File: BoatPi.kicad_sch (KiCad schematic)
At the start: 57 parts, among them J1 1432431, J10 CONSMA002-SMD-G, J11 CONSMA002-SMD-G, J12 CONSMA002-SMD-G, J14 Barrel_Jack_MountingPin, J2 1436987, J4 JAE_SIM_Card_SF72S006, J7 1436987, J8 1432431, M2 Fan_CPU_4pin, U1 SIM7600E-H, U10 AP62301WU-7, U2 PC817, U3 PC817, U4 PC817, U5 PC817, U6 PC817, U7 PC817, U8 PC817, U9 PC817

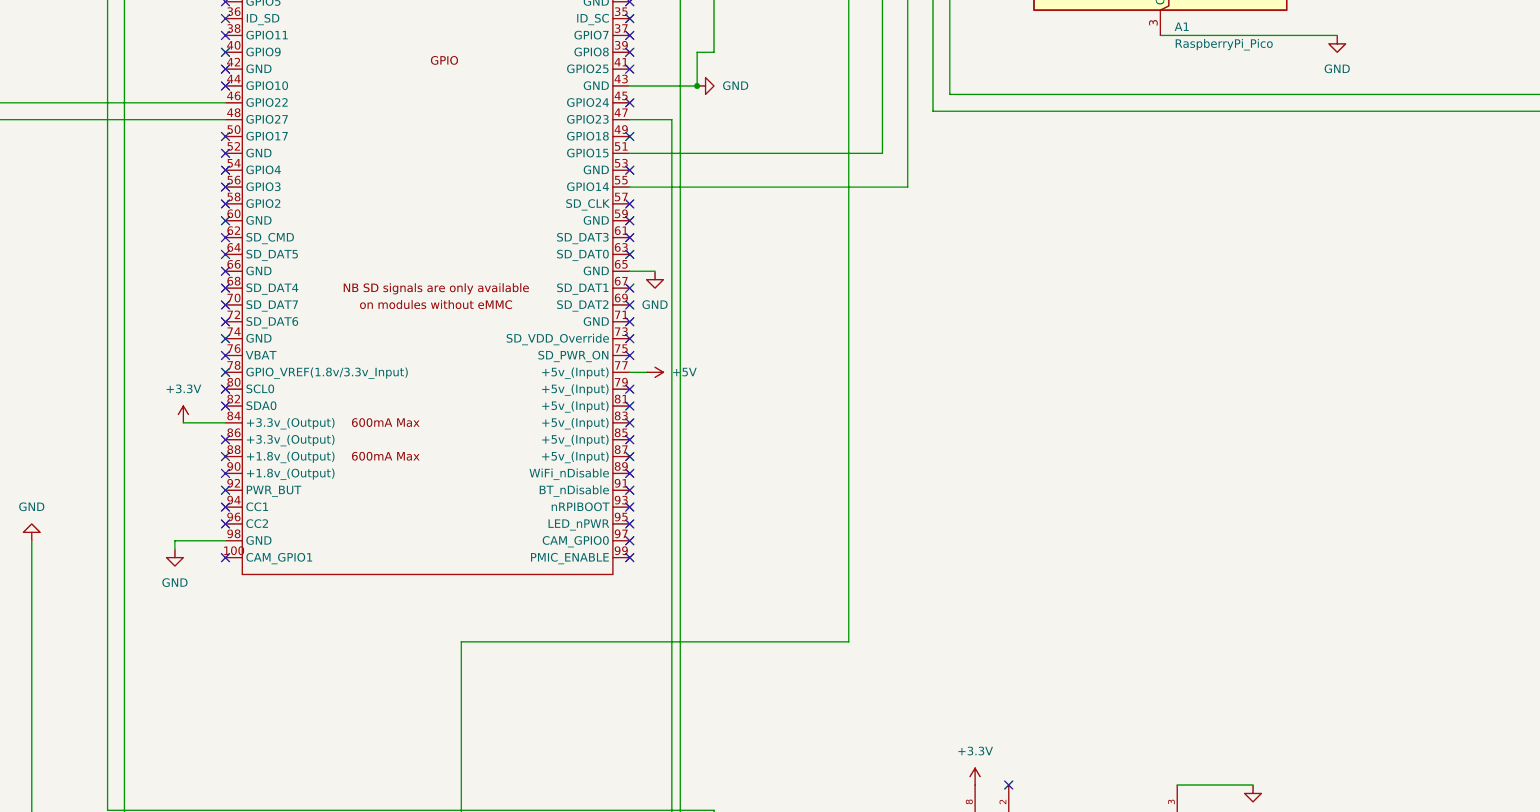
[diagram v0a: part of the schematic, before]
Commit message: Home push
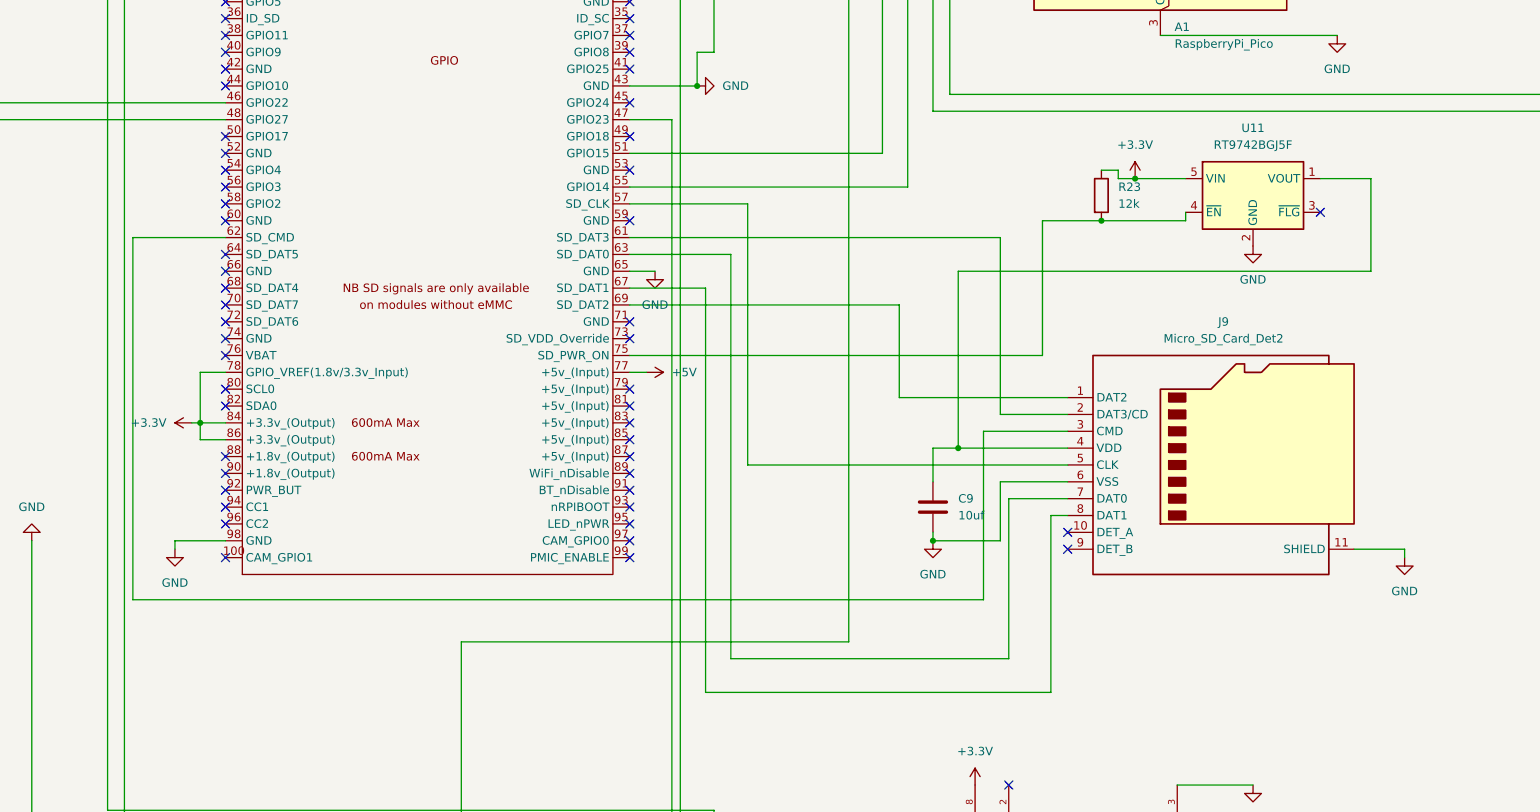
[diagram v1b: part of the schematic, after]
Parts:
- added C9: 10uf, Capacitor_SMD:C_0805_2012Metric, symbol Device:C
- added J9: Micro_SD_Card_Det2, Connector_Card:SD_TE_2041021, symbol Connector:Micro_SD_Card_Det2
- added R23: 12k, Resistor_SMD:R_0805_2012Metric, symbol Device:R
- added U11: RT9742BGJ5F, Package_TO_SOT_SMD:TSOT-23-5, symbol Power_Management:RT9742BGJ5F
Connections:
- net +3.3V: now also Module1.78 (GPIO_VREF(1.8v/3.3v_Input)), Module1.86 (+3.3v_(Output)), R23.1, U11.5 (VIN)
- net GND: now also C9.2, J9.11 (SHIELD), J9.6 (VSS), U11.2 (GND)
- net at Module1.57 (SD_CLK): now also J9.5 (CLK)
- net at Module1.61 (SD_DAT3): now also J9.2 (DAT3/CD)
- net at Module1.62 (SD_CMD): now also J9.3 (CMD)
- net at Module1.63 (SD_DAT0): now also J9.7 (DAT0)
- net at Module1.67 (SD_DAT1): now also J9.8 (DAT1)
- net at Module1.69 (SD_DAT2): now also J9.1 (DAT2)
- net at Module1.75 (SD_PWR_ON): now also R23.2, U11.4 (~{EN})
- new net: C9.1, J9.4 (VDD), U11.1 (VOUT)
- no-connect marks 190 -> 184

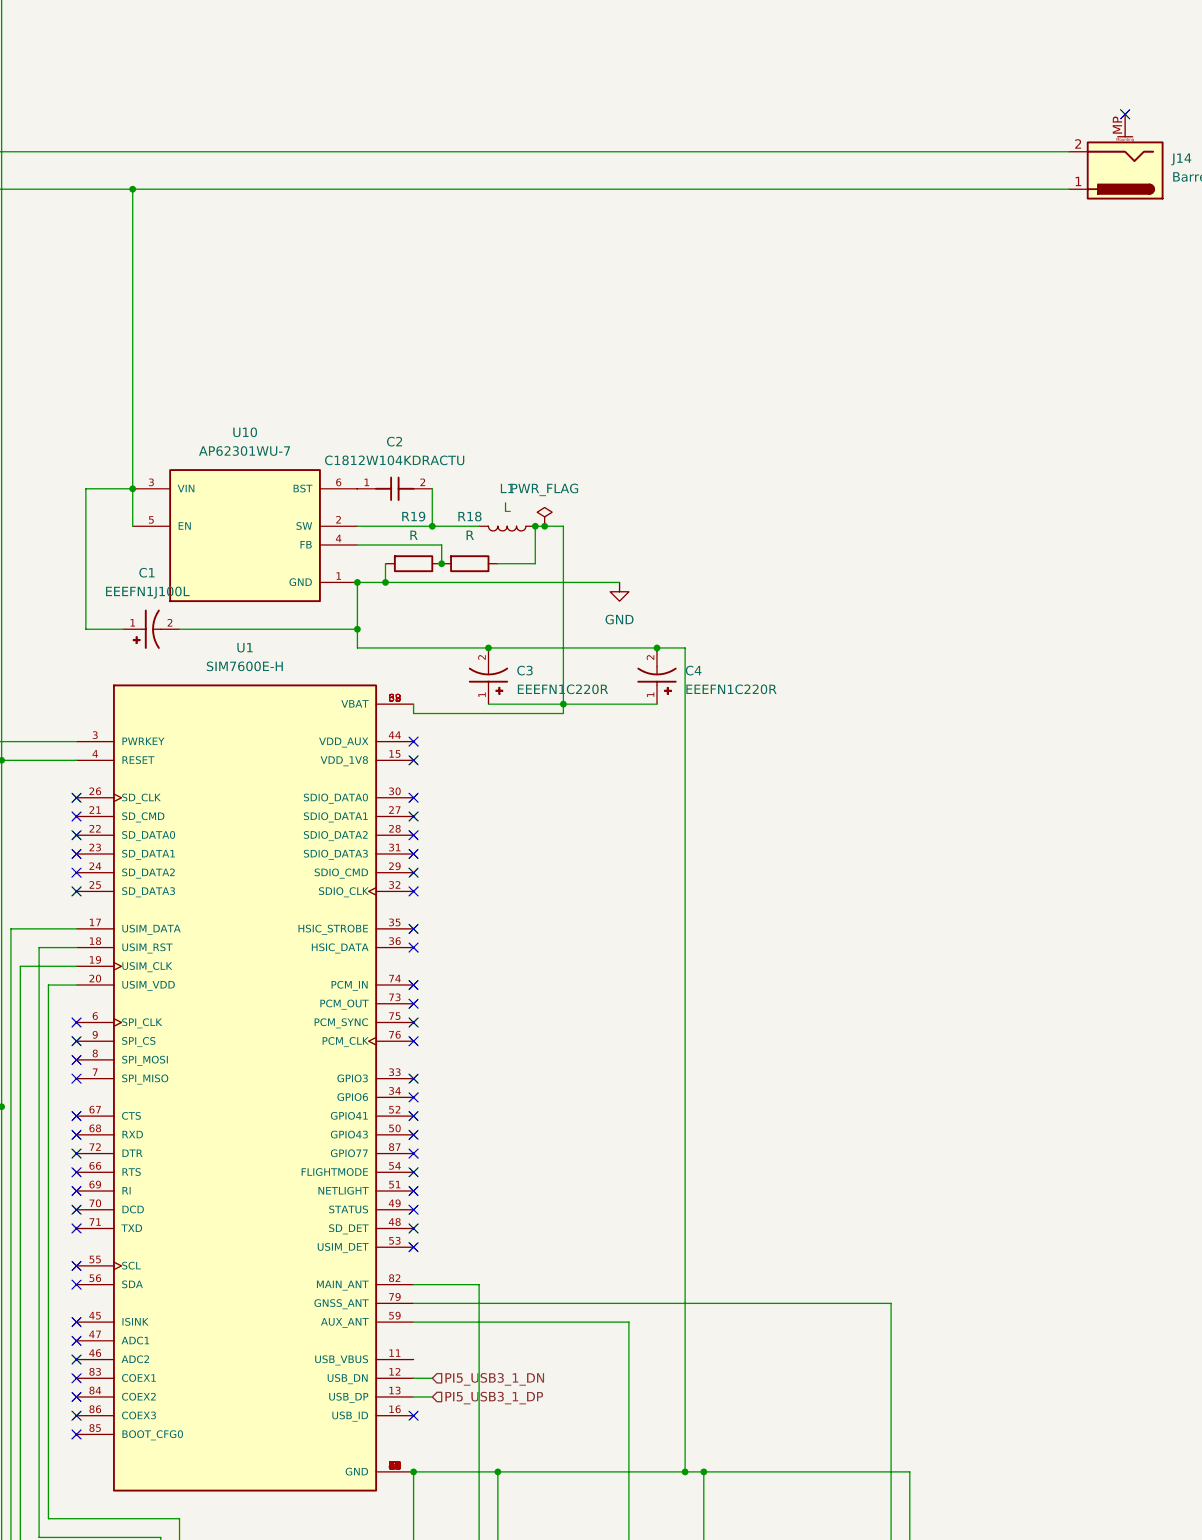
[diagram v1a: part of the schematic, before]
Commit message: Work Changes and documentation
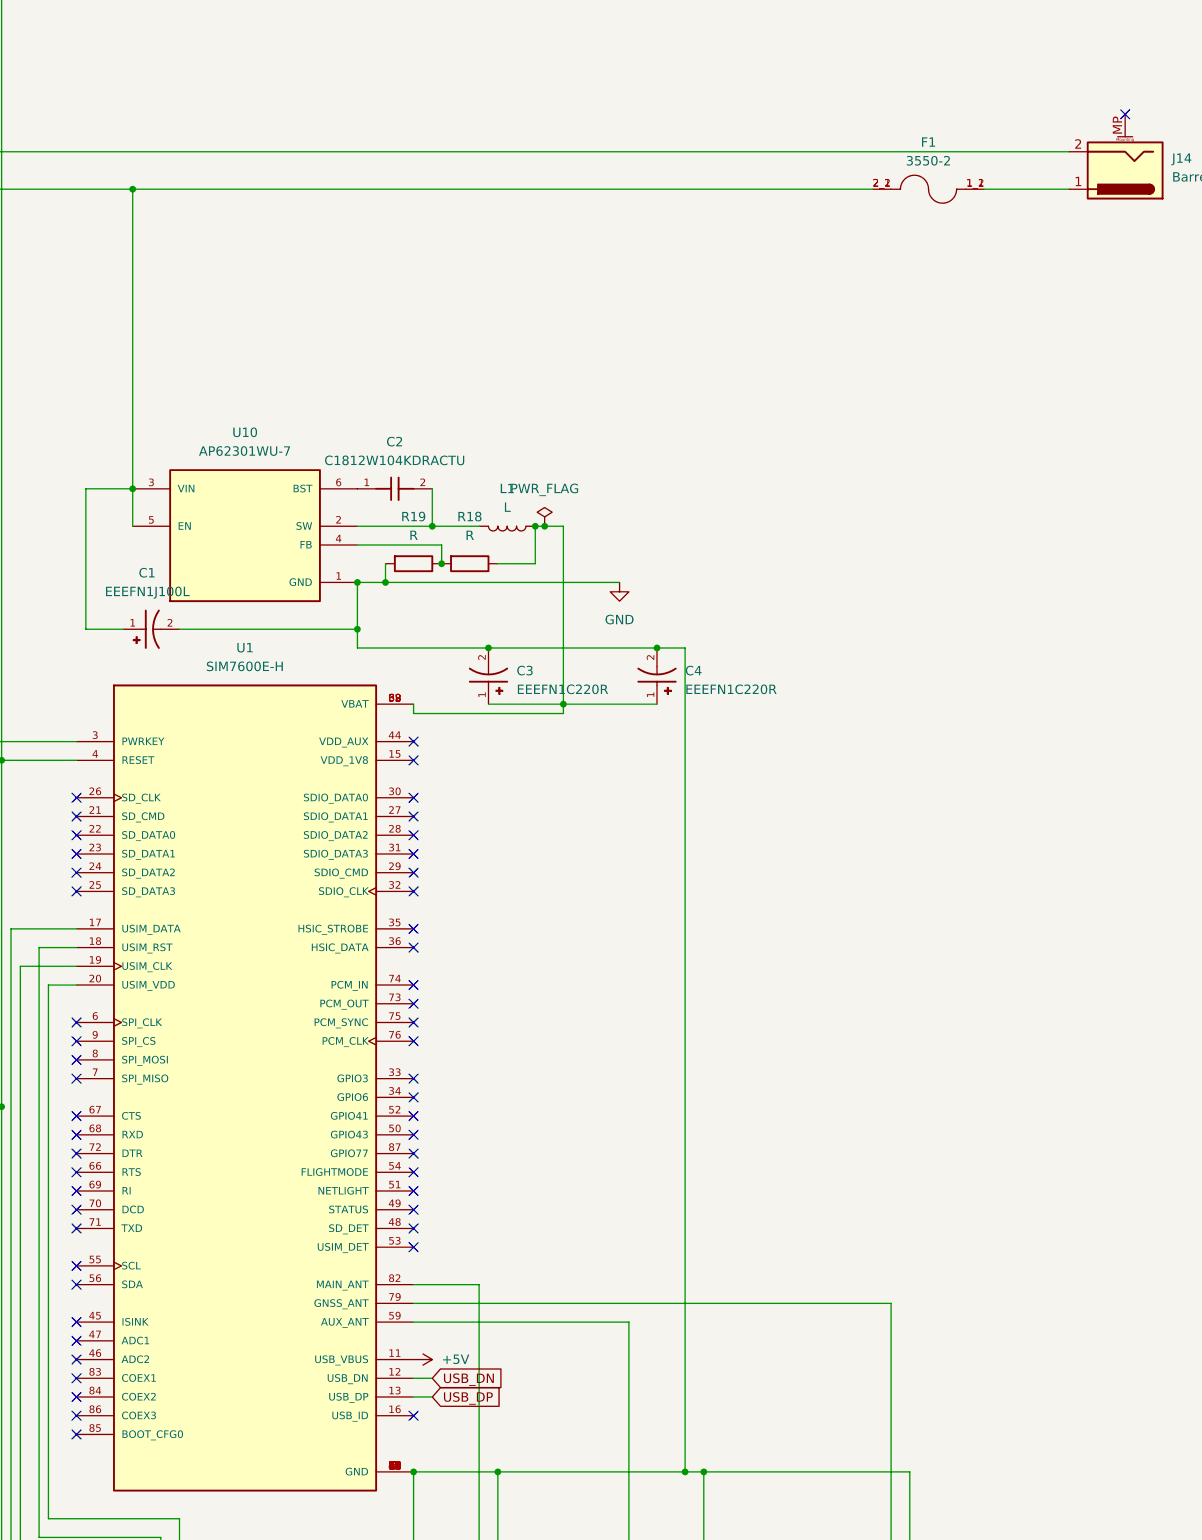
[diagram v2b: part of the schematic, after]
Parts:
- added F1: 3550-2, NewFuseHolderPretty:FUSE_3550-2, symbol NewFuseHolder:3550-2
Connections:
- net +5V: now also U1.11 (USB_VBUS)
- net at C1.1, C7.1, C8.1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: now also F1.2_1, F1.2_2; no longer J14.1
- net PI5_USB3_1_DN renamed USB_DN
- net PI5_USB3_1_DP renamed USB_DP
- new net: F1.1_1, F1.1_2, J14.1
